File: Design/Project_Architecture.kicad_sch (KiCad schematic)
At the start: 0 parts

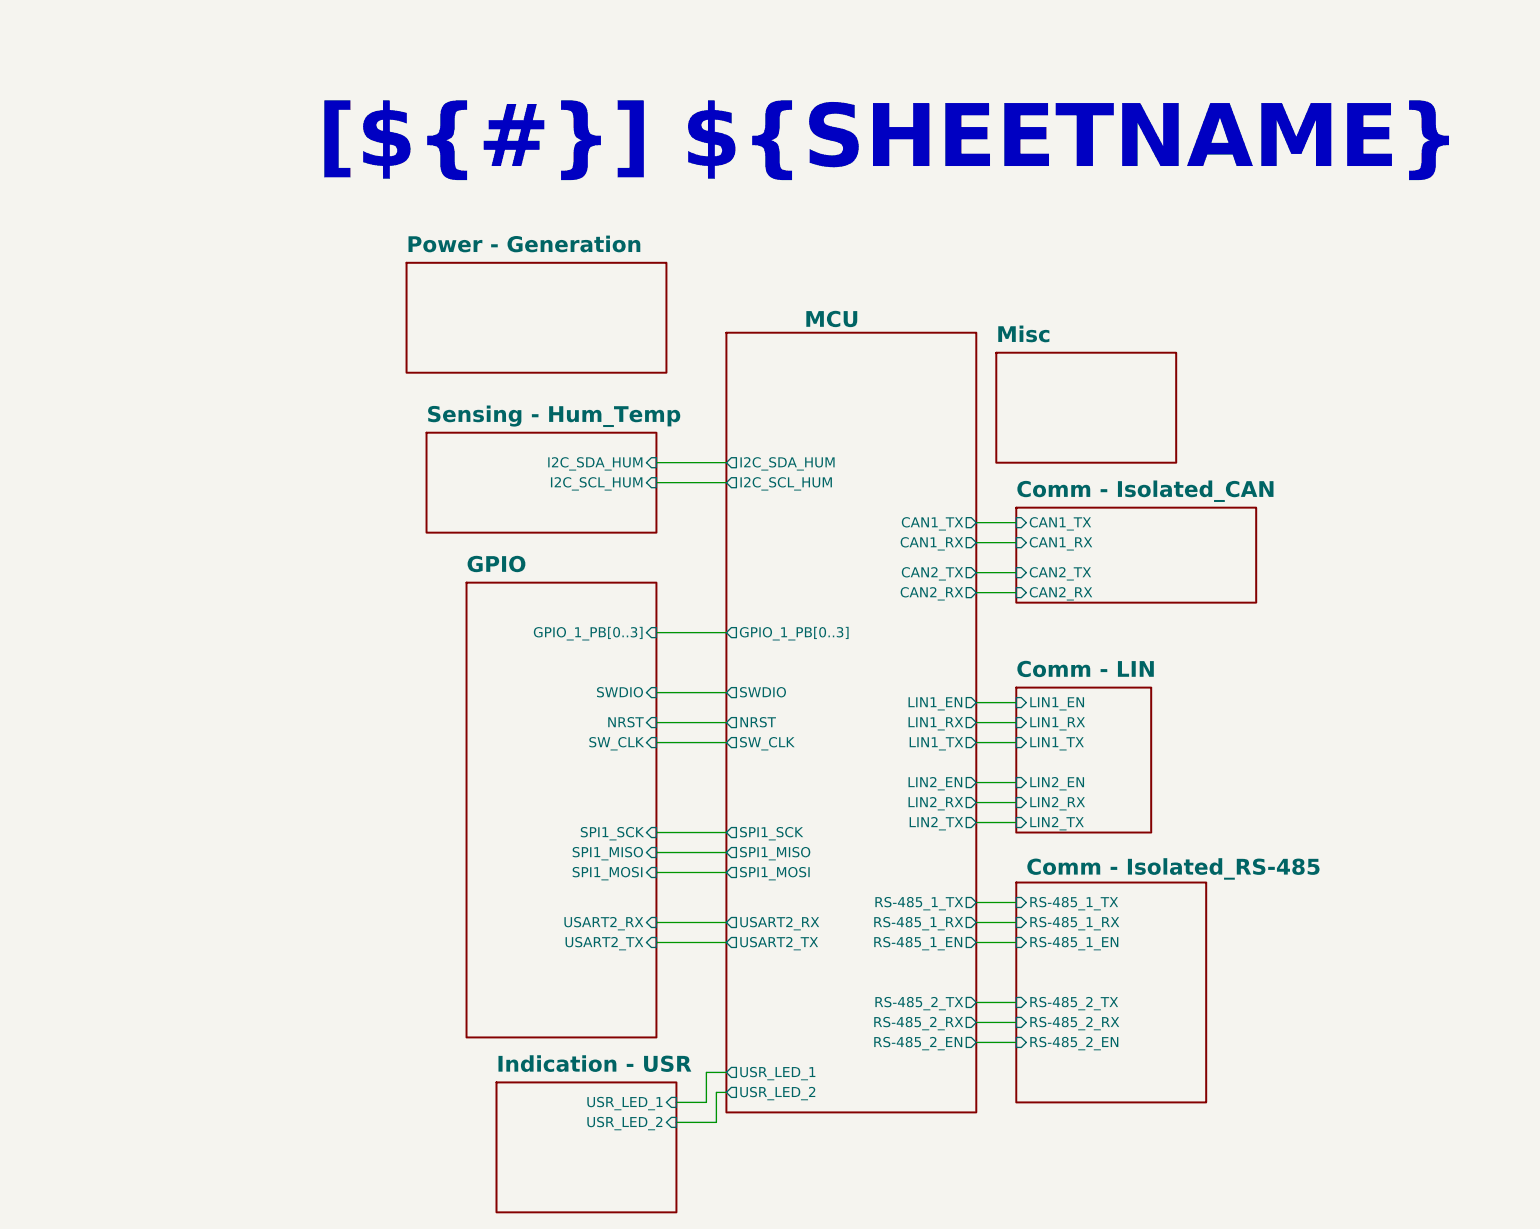
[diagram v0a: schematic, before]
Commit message: new Design for Prototyping
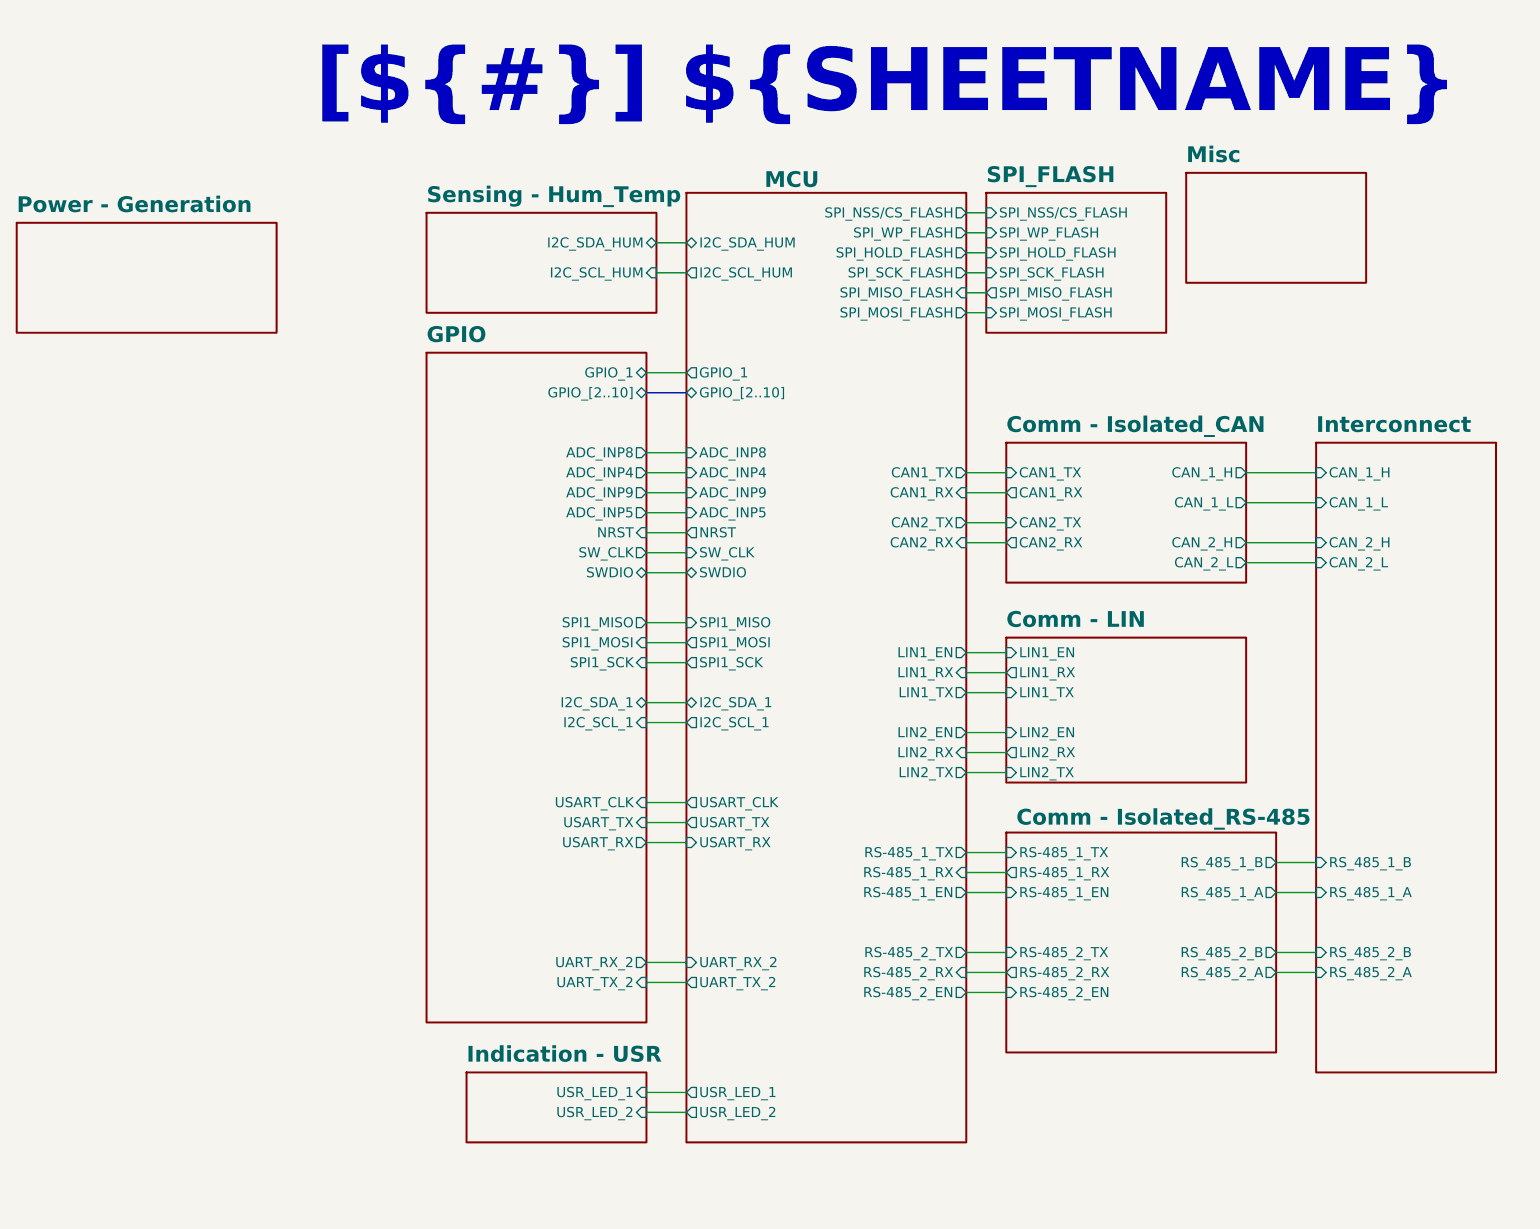
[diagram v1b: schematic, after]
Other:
- added sheet Interconnect (Interconnect.kicad_sch)
- added sheet SPI_FLASH (SPI_FLASH.kicad_sch)
- sheet Comm - Isolated_CAN ports: added CAN_1_H, CAN_1_L, CAN_2_H, CAN_2_L; removed none
- sheet Comm - Isolated_RS-485 ports: added RS_485_1_A, RS_485_1_B, RS_485_2_A, RS_485_2_B; removed none
- sheet GPIO ports: added ADC_INP4, ADC_INP5, ADC_INP8, ADC_INP9, GPIO_1, GPIO_[2..10], I2C_SCL_1, I2C_SDA_1, UART_RX_2, UART_TX_2, USART_CLK, USART_RX, USART_TX; removed GPIO_1_PB[0..3], USART2_RX, USART2_TX
- sheet MCU ports: added ADC_INP4, ADC_INP5, ADC_INP8, ADC_INP9, GPIO_1, GPIO_[2..10], I2C_SCL_1, I2C_SDA_1, SPI_HOLD_FLASH, SPI_MISO_FLASH, SPI_MOSI_FLASH, SPI_NSS/CS_FLASH, SPI_SCK_FLASH, SPI_WP_FLASH, UART_RX_2, UART_TX_2, USART_CLK, USART_RX, USART_TX; removed GPIO_1_PB[0..3], USART2_RX, USART2_TX
- title: Rapid-Core -> (none)
